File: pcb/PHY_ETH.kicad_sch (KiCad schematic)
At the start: 15 parts, among them U1 LAN8742A, Y1 LFXTAL071758Cutt

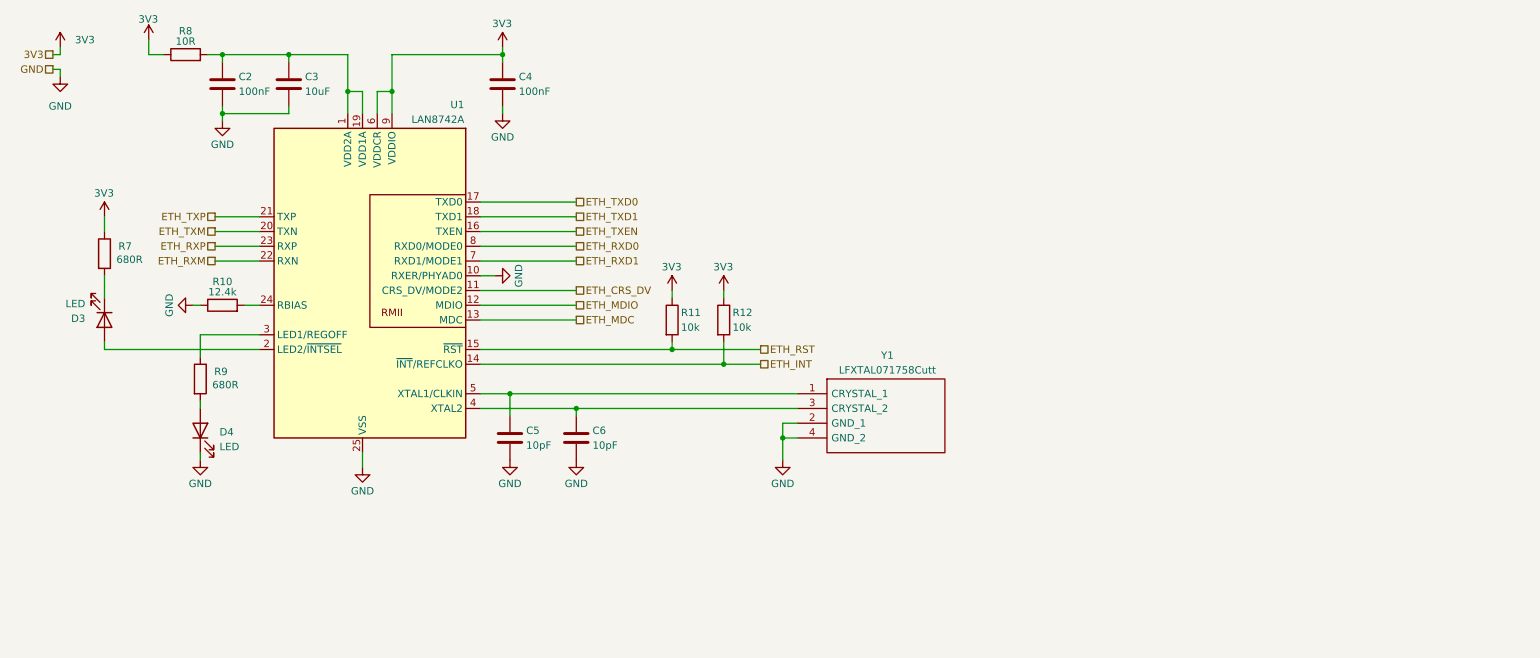
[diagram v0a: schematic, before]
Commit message: updated ethernet
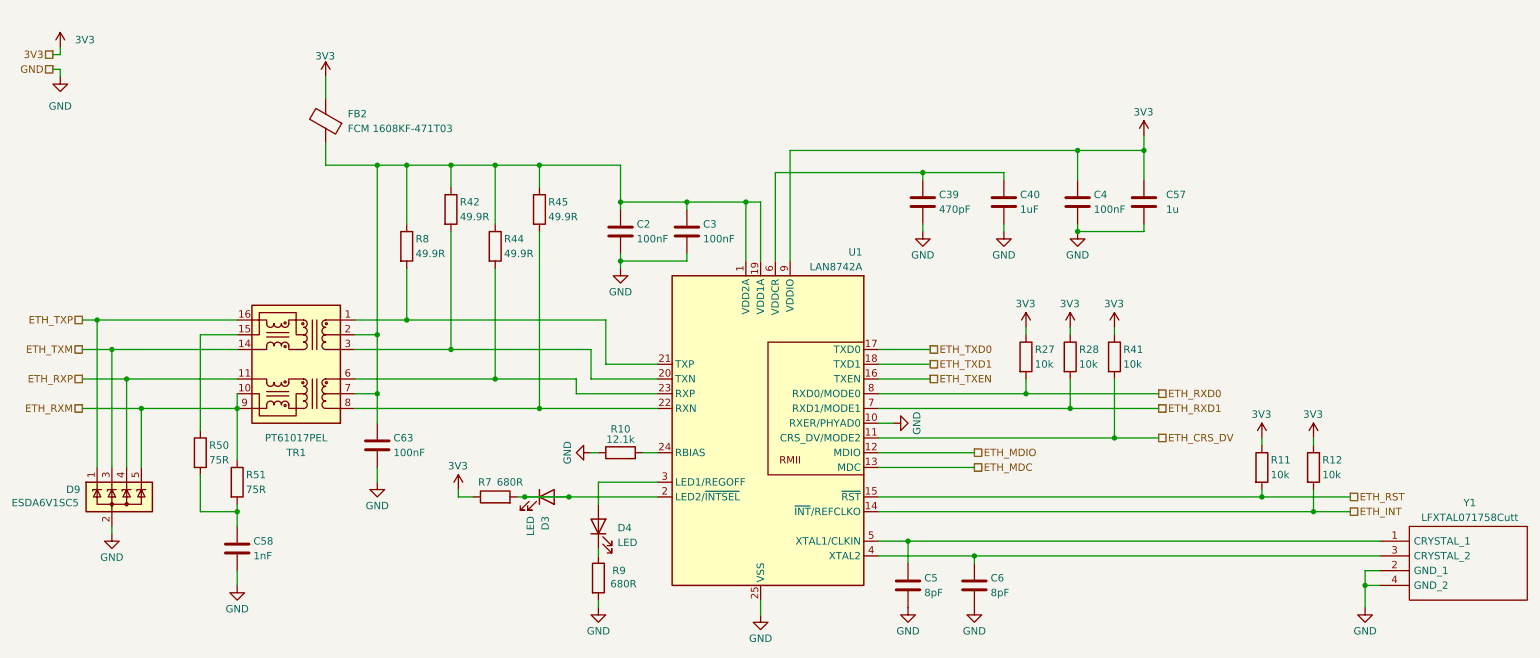
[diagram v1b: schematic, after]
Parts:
- added C39: 470pF, Capacitor_SMD:C_0603_1608Metric_Pad1.08x0.95mm_HandSolder, symbol Device:C
- added C40: 1uF, Capacitor_SMD:C_0603_1608Metric_Pad1.08x0.95mm_HandSolder, symbol Device:C
- added C57: 1u, Capacitor_SMD:C_0603_1608Metric, symbol Device:C
- added C58: 1nF, Capacitor_SMD:C_0603_1608Metric_Pad1.08x0.95mm_HandSolder, symbol Device:C
- added C63: 100nF, Capacitor_SMD:C_0603_1608Metric_Pad1.08x0.95mm_HandSolder, symbol Device:C
- added D9: ESDA6V1SC5, Package_TO_SOT_SMD:SOT-23-5, symbol Power_Protection:ESDA6V1SC5
- added FB2: FCM 1608KF-471T03, Inductor_SMD:L_0603_1608Metric_Pad1.05x0.95mm_HandSolder, symbol Device:FerriteBead
- added R27, R28, R41: 10k, Resistor_SMD:R_0603_1608Metric_Pad0.98x0.95mm_HandSolder, symbol Device:R
- added R42, R44, R45: 49.9R, Resistor_SMD:R_0603_1608Metric_Pad0.98x0.95mm_HandSolder, symbol Device:R
- added R50, R51: 75R, Resistor_SMD:R_0603_1608Metric_Pad0.98x0.95mm_HandSolder, symbol Device:R
- added TR1: PT61017PEL, Transformer_SMD:Transformer_Ethernet_Bourns_PT61017PEL, symbol Transformer:PT61017PEL
- C3: value 10uF -> 100nF
- C5, C6: value 10pF -> 8pF
- R10: value 12.4k -> 12.1k
- R8: value 10R -> 49.9R
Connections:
- net 3V3: now also C57.1, FB2.2, R27.1, R28.1, R41.1; no longer R8.1, U1.6 (VDDCR)
- net ETH_CRS_DV: now also R41.2
- net ETH_RXD0: now also R27.2
- net ETH_RXD1: now also R28.2
- net ETH_RXM: now also D9.5 (K), R51.1, TR1.10 (C_RX), TR1.9 (RX-); no longer U1.22 (RXN)
- net ETH_RXP: now also D9.4 (K), TR1.11 (RX+); no longer U1.23 (RXP)
- net ETH_TXM: now also D9.3 (K), TR1.14 (TX-); no longer U1.20 (TXN)
- net ETH_TXP: now also D9.1 (K), TR1.16 (TX+); no longer U1.21 (TXP)
- net GND: now also R9.2, C39.2, C40.2, C57.2, C58.2, C63.2, D9.2 (A); no longer D4.1 (K)
- net at D3.1 (K), R7.2: now also D3.2 (A), U1.2 (LED2/~{INTSEL})
- net at D4.2 (A): now also U1.3 (LED1/REGOFF); no longer R9.2
- net at R9.1: now also D4.1 (K); no longer U1.3 (LED1/REGOFF)
- net at C2.1, C3.1, U1.1 (VDD2A)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: now also R8.1, C63.1, FB2.1, R42.1, R44.1, R45.1, TR1.2 (C_TD), TR1.7 (C_RD); no longer R8.2
- new net: C58.1, R50.2, R51.2
- new net: R42.2, TR1.3 (TD-), U1.20 (TXN)
- new net: R8.2, TR1.1 (TD+), U1.21 (TXP)
- new net: R45.2, TR1.8 (RD-), U1.22 (RXN)
- new net: R44.2, TR1.6 (RD+), U1.23 (RXP)
- new net: C39.1, C40.1, U1.6 (VDDCR)
- new net: R50.1, TR1.15 (C_TX)
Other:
- moved on the sheet: C2, C3, C4, C5, C6, D3, D4, R10, R11, R12, R7, R9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
